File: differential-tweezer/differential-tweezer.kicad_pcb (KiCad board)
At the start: 4 copper layers, 32 x 23 mm, 64 parts, among them J1 5V, J2 IN+, J3 Conn_Coaxial, J4 IN-, J5 Power, U1 R1283B, U2 OPA810, U3 OPA810, U4 OPA810

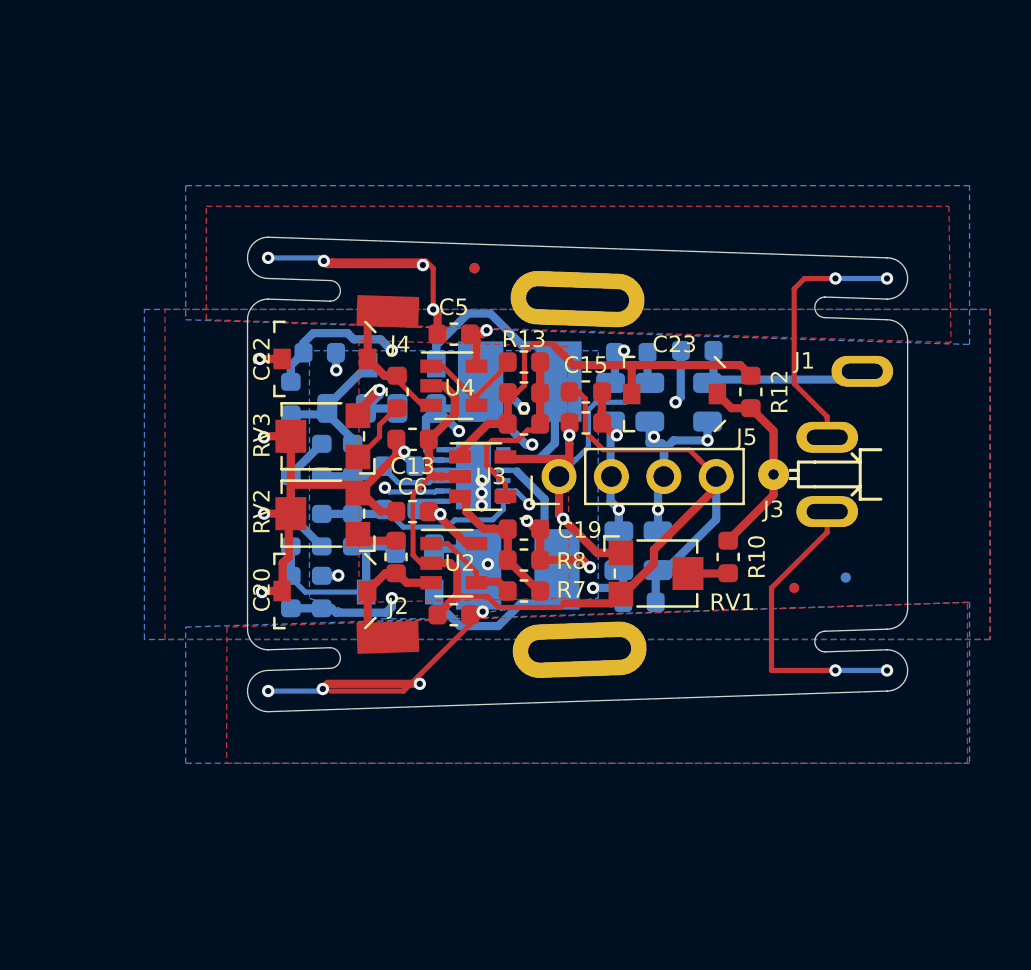
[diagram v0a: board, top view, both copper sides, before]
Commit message: Revision 2
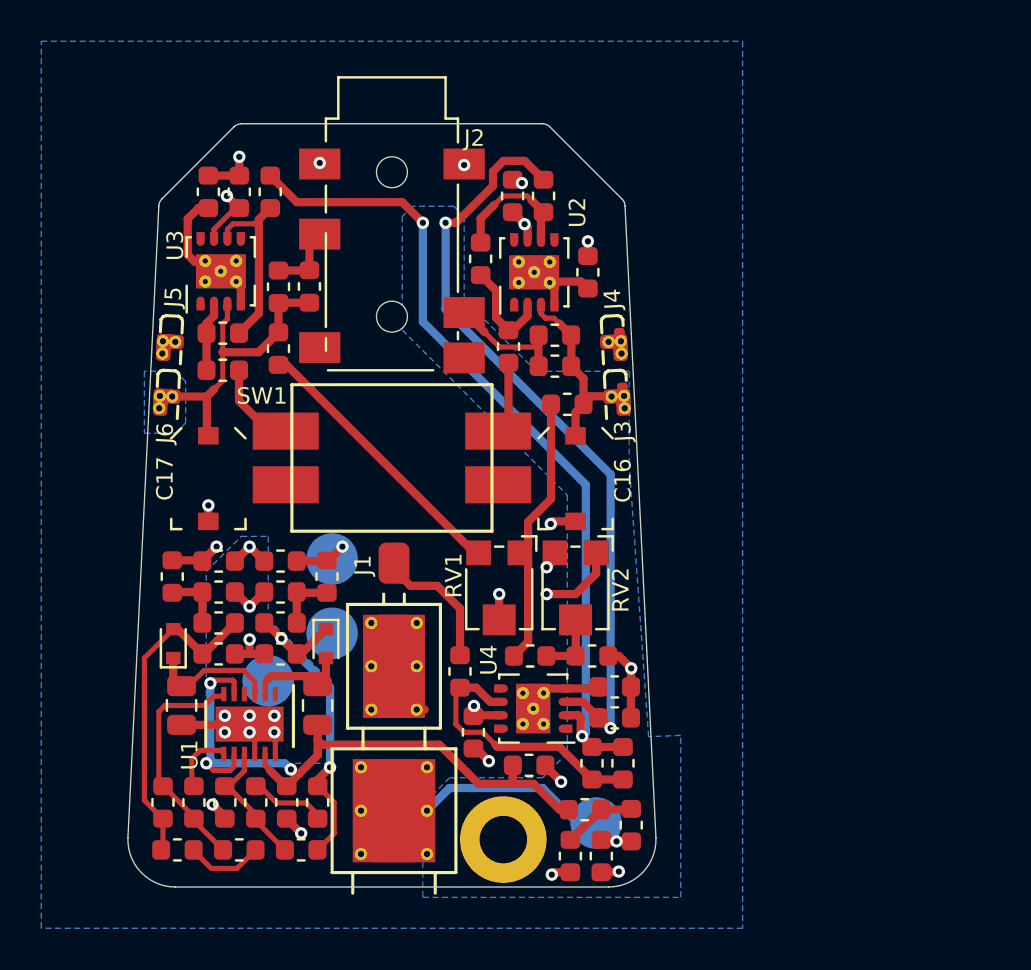
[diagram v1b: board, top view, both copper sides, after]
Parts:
- removed C11: 100nF, Capacitor_SMD:C_0603_1608Metric
- removed C18: 22nF, Capacitor_SMD:C_0603_1608Metric
- removed FID1, FID2, FID3, FID4: Fiducial_0.5mm_Mask1mm, Fiducial:Fiducial_0.5mm_Mask1mm
- removed R8: 470, Resistor_SMD:R_0603_1608Metric
- removed RV3: 47k, Potentiometer_SMD:Potentiometer_Bourns_TC33X_Vertical
- removed SLOT1, SLOT2: SLOT_5x1, oscilloscope-probes:SLOT_5x1
- added C24: 100nF, Capacitor_SMD:C_0603_1608Metric, F.Cu at (88.0, 144.5)
- added C25: 100nF, Capacitor_SMD:C_0603_1608Metric, F.Cu at (94.8, 142.3)
- added C26: 10µF, Capacitor_SMD:C_0603_1608Metric, F.Cu at (78.9, 147.9)
- added H1: 2.2mm, MountingHole:MountingHole_2.2mm_M2_DIN965_Pad, F.Cu at (89.4, 149.7)
- added J6: Probe-, oscilloscope-probes:TE_2306454_LEFT, F.Cu at (72.9, 128.2)
- added L8: 1k, Inductor_SMD:L_0603_1608Metric, F.Cu at (73.3, 136.9)
- added R16: 22, Resistor_SMD:R_0603_1608Metric, F.Cu at (89.7, 125.8)
- added R17: 22, Resistor_SMD:R_0603_1608Metric, F.Cu at (75.8, 127.0)
- added R18: 110, Resistor_SMD:R_0603_1608Metric, F.Cu at (91.3, 118.5)
- added R19: 110, Resistor_SMD:R_0603_1608Metric, F.Cu at (78.1, 118.3)
- added R20: 220, Resistor_SMD:R_0603_1608Metric, F.Cu at (94.8, 143.8)
- added R21: 220, Resistor_SMD:R_0603_1608Metric, F.Cu at (93.7, 146.0)
- added R22: 49.9, Resistor_SMD:R_0603_1608Metric, F.Cu at (87.3, 141.6)
- added SW1: GAIN, oscilloscope-probes:78HF01GWRT, F.Cu at (84.0, 131.2)
- added TP1: +5V, TestPoint:TestPoint_Pad_D2.5mm, B.Cu at (93.9, 148.9)
- added TP2: +6V, TestPoint:TestPoint_Pad_D2.5mm, B.Cu at (81.1, 136.1)
- added TP3: -6V, TestPoint:TestPoint_Pad_D2.5mm, B.Cu at (81.1, 139.7)
- added TP4: GND, TestPoint:TestPoint_Pad_D2.5mm, B.Cu at (78.0, 142.0)
- C1, C12, C2, C9: footprint Capacitor_SMD:C_0805_2012Metric -> Capacitor_SMD:C_0603_1608Metric; moved to F.Cu
- C10: value 10µF -> 100nF; footprint Capacitor_SMD:C_0805_2012Metric -> Capacitor_SMD:C_0603_1608Metric; moved to F.Cu
- C13, C6, C7: value 100nF -> 10µF
- C14, C15: value 100nF -> 20pF
- C16, C17: value 10µF -> 8-30pF; footprint Capacitor_SMD:C_0805_2012Metric -> Capacitor_SMD:C_Trimmer_Murata_TZC3; moved to F.Cu
- C19: value 2pF -> N/A
- C20, C22, C23: value 6pF -> 100nF; footprint Capacitor_SMD:C_Trimmer_Murata_TZC3 -> Capacitor_SMD:C_0603_1608Metric
- C21: value 2pF -> 100nF
- C3: value 100nF -> 10µF; moved to F.Cu
- C4: value 10µF -> 100pF; footprint Capacitor_SMD:C_0805_2012Metric -> Capacitor_SMD:C_0603_1608Metric; moved to F.Cu
- C5: value 100nF -> 100pF
- C8: value 22nF -> 10µF; moved to F.Cu
- D1, D2: value BAT54 -> NSR05T30; footprint Diode_SMD:D_SOD-123 -> Diode_SMD:D_SOD-523; moved to F.Cu
- J1: value 5V -> Triax; footprint oscilloscope-probes:WIREPAD_WIDE -> oscilloscope-probes:TRIAX_TUBE
- J2: value IN+ -> Input; footprint oscilloscope-probes:SOLDERPAD_3x1.5 -> oscilloscope-probes:Tensility_54-00177
- J3: value Conn_Coaxial -> Probe+; footprint oscilloscope-probes:COAX_SOLDER -> oscilloscope-probes:TE_2306454_RIGHT
- J4: value IN- -> Probe+_GND; footprint oscilloscope-probes:SOLDERPAD_3x1.5 -> oscilloscope-probes:TE_2306454_RIGHT
- J5: value Power -> Probe-_GND; footprint Connector_PinHeader_2.54mm:PinHeader_1x04_P2.54mm_Vertical -> oscilloscope-probes:TE_2306454_LEFT
- L1, L5, L6, R1, R4, U1: moved to F.Cu
- L2, L7: value 47µH -> 1k; footprint Inductor_SMD:L_Taiyo-Yuden_NR-40xx_HandSoldering -> Inductor_SMD:L_0603_1608Metric; moved to F.Cu
- L3, L4: value 1k -> 4.7µH; footprint Inductor_SMD:L_0603_1608Metric -> Inductor_SMD:L_0805_2012Metric; moved to F.Cu
- R10, R9: value 1M -> 499k
- R12: value 47 -> 475k
- R13: value 470 -> 475k
- R14: value 470 -> 220
- R15: value 1M -> 220
- R2: value 100k -> 4.99k; moved to F.Cu
- R3: value 10k -> 4.99k; moved to F.Cu
- R5: value 100k -> 1k; moved to F.Cu
- R6: value 10k -> 1k; moved to F.Cu
- R7: value 470 -> 10M
- RV1, RV2: value 47k -> 50k
- U2, U3, U4: value OPA810 -> OPA659; footprint Package_TO_SOT_SMD:SOT-23-5 -> Package_SON:Texas_S-PVSON-N8_ThermalVias
- moved L4 27.7 mm to (73.8, 143.2), turned to 90 degrees
- moved C4 27.2 mm to (77.4, 147.9)
- moved C5 27.1 mm to (76.6, 150.2)
- moved J1 26.1 mm to (84.1, 139.8), turned to 90 degrees
- moved C1 25.0 mm to (94.2, 150.5), turned to 270 degrees
- moved C23 24.6 mm to (75.1, 118.3), turned to 270 degrees
- moved R10 24.2 mm to (80.0, 122.9)
- moved L1 23.2 mm to (95.6, 149.0), turned to 90 degrees
- moved C3 22.4 mm to (90.7, 146.1)
- moved C2 22.1 mm to (92.7, 150.5)
- moved C20 21.2 mm to (89.8, 118.5), turned to 90 degrees
- moved C7 21.0 mm to (75.6, 140.7)
- moved L2 21.0 mm to (93.3, 148.2), turned to 180 degrees
- moved L6 20.4 mm to (75.6, 139.2), turned to 180 degrees
- moved J5 20.1 mm to (73.0, 125.5), turned to 87 degrees
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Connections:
- C1 pad 1: Net-(C1-Pad1) -> +5V
- C10 pad 1: Net-(C10-Pad1) -> /OFFSET_TRIM
- C12 pad 1: -12V -> +6V
- C13 pad 1: GND -> -6V
- C13 pad 2: -12V -> GND
- C14 pad 1: GND -> /IN+
- C14 pad 2: -12V -> /CONN_IN+
- C15 pad 1: GND -> /IN-
- C15 pad 2: -12V -> /CONN_IN-
- C16 pad 1: Net-(C16-Pad1) -> /IN+
- C17 pad 1: Net-(C17-Pad1) -> /IN-
- C19 pad 1: GND -> Net-(C19-Pad1)
- C20 pad 1: Net-(C20-Pad1) -> +6V
- C21 pad 1: Net-(C21-Pad1) -> GND
- C21 pad 2: Net-(C21-Pad2) -> -6V
- C22 pad 1: Net-(C22-Pad1) -> +6V
- C23 pad 1: Net-(C23-Pad1) -> GND
- C23 pad 2: Net-(C21-Pad1) -> -6V
- C3 pad 1: Net-(C2-Pad1) -> Net-(C26-Pad1)
- C4 pad 1: +12V -> Net-(C4-Pad1)
- C4 pad 2: GND -> Net-(C4-Pad2)
- C5 pad 1: +12V -> Net-(C5-Pad1)
- C5 pad 2: GND -> Net-(C5-Pad2)
- C6 pad 1: +12V -> Net-(C6-Pad1)
- C7 pad 1: +12V -> Net-(C7-Pad1)
- C8 pad 2: Net-(C8-Pad2) -> GND
- D1 pad 1: Net-(C1-Pad1) -> Net-(D1-Pad1)
- D1 pad 2: Net-(D1-Pad2) -> Net-(C7-Pad1)
- D2 pad 1: Net-(D2-Pad1) -> Net-(C6-Pad1)
- D2 pad 2: Net-(C9-Pad1) -> Net-(D2-Pad2)
- J1 pad 1: Net-(C16-Pad1) -> /OUT
- J3 pad 1: Net-(C23-Pad1) -> /IN+
- J4 pad 1: Net-(C22-Pad1) -> GND
- J5 pad 1: +12V -> GND
- L1 pad 1: Net-(C16-Pad1) -> +5V
- L1 pad 2: Net-(C17-Pad1) -> Net-(C2-Pad1)
- L2 pad 1: Net-(C17-Pad1) -> Net-(C2-Pad1)
- L2 pad 2: Net-(D1-Pad2) -> Net-(C26-Pad1)
- L3 pad 1: Net-(C1-Pad1) -> Net-(C26-Pad1)
- L3 pad 2: Net-(C2-Pad1) -> Net-(D2-Pad2)
- L4 pad 1: Net-(C2-Pad1) -> GND
- L4 pad 2: +12V -> Net-(D1-Pad1)
- L5 pad 1: Net-(C9-Pad1) -> Net-(C6-Pad1)
- L5 pad 2: Net-(C10-Pad1) -> Net-(C8-Pad1)
- L6 pad 1: Net-(C10-Pad1) -> Net-(C7-Pad1)
- L6 pad 2: -12V -> Net-(C9-Pad1)
- L7 pad 1: GND -> Net-(C8-Pad1)
- L7 pad 2: Net-(D2-Pad1) -> +6V
- R1 pad 1: Net-(C8-Pad1) -> Net-(C5-Pad2)
- R1 pad 2: Net-(C1-Pad1) -> Net-(R1-Pad2)
- R10 pad 1: Net-(R10-Pad1) -> /IN-
- R10 pad 2: Net-(C23-Pad1) -> /CONN_IN-
- R12 pad 1: Net-(C23-Pad1) -> /IN+
- R12 pad 2: Net-(C21-Pad1) -> Net-(R12-Pad2)
- R13 pad 1: Net-(R13-Pad1) -> /IN-
- R13 pad 2: Net-(C21-Pad2) -> Net-(R13-Pad2)
- R14 pad 1: Net-(C21-Pad2) -> Net-(R14-Pad1)
- R14 pad 2: Net-(C21-Pad1) -> Net-(R14-Pad2)
- R15 pad 1: Net-(C22-Pad1) -> Net-(R15-Pad1)
- R2 pad 1: Net-(C1-Pad1) -> Net-(C6-Pad1)
- R2 pad 2: Net-(C8-Pad2) -> Net-(C4-Pad2)
- R3 pad 1: GND -> Net-(C7-Pad1)
- R3 pad 2: Net-(C8-Pad2) -> Net-(C5-Pad2)
- R4 pad 1: Net-(C18-Pad1) -> Net-(C4-Pad1)
- R4 pad 2: Net-(C9-Pad1) -> Net-(C6-Pad1)
- R5 pad 1: Net-(C9-Pad1) -> Net-(C5-Pad1)
- R5 pad 2: Net-(C18-Pad2) -> Net-(C7-Pad1)
- R6 pad 1: Net-(C18-Pad2) -> GND
- R6 pad 2: Net-(R6-Pad2) -> Net-(C4-Pad2)
- R7 pad 1: Net-(R7-Pad1) -> /OFFSET_TRIM
- R7 pad 2: Net-(C19-Pad2) -> Net-(R12-Pad2)
- R9 pad 1: Net-(C20-Pad1) -> /IN+
- R9 pad 2: Net-(R9-Pad2) -> /CONN_IN+
- RV1 pad 1: +12V -> Net-(R12-Pad2)
- RV1 pad 2: Net-(R10-Pad1) -> GND
- RV1 pad 3: -12V -> Net-(R13-Pad2)
- RV2 pad 1: Net-(R9-Pad2) -> +6V
- RV2 pad 2: GND -> /OFFSET_TRIM
- RV2 pad 3: GND -> -6V
- U1 pad 11: Net-(C17-Pad1) -> Net-(C26-Pad1)
- U1 pad 2: Net-(D1-Pad2) -> Net-(D2-Pad2)
- U1 pad 3: Net-(D2-Pad1) -> Net-(D1-Pad1)
- U1 pad 5: Net-(C17-Pad1) -> Net-(C26-Pad1)
- U1 pad 6: Net-(C18-Pad2) -> Net-(C5-Pad2)
- U1 pad 7: Net-(R6-Pad2) -> Net-(R1-Pad2)
- U1 pad 8: Net-(C17-Pad1) -> Net-(C26-Pad1)
- U1 pad 9: Net-(C8-Pad2) -> Net-(C4-Pad2)
- U2 pad 1: Net-(R7-Pad1) -> Net-(U2-Pad1)
- U2 pad 2: -12V -> Net-(R14-Pad2)
- U2 pad 3: Net-(C20-Pad1) -> /IN+
- U2 pad 4: Net-(R7-Pad1) -> -6V
- U2 pad 5: +12V -> Net-(U2-Pad5)
- U3 pad 1: Net-(C21-Pad1) -> Net-(U3-Pad1)
- U3 pad 2: -12V -> Net-(R15-Pad1)
- U3 pad 3: Net-(C19-Pad2) -> /IN-
- U3 pad 4: Net-(C21-Pad2) -> -6V
- U3 pad 5: +12V -> Net-(U3-Pad5)
- U4 pad 1: Net-(R13-Pad1) -> Net-(U4-Pad1)
- U4 pad 2: -12V -> Net-(C19-Pad2)
- U4 pad 3: Net-(C22-Pad1) -> Net-(R18-Pad2)
- U4 pad 4: Net-(R13-Pad1) -> -6V
- U4 pad 5: +12V -> Net-(U4-Pad5)
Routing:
- net GND: track 131.9 -> 34.9 mm, vias 31 -> 24
- net -12V: track 50.4 -> 0.00 mm
- net +12V: track 40.2 -> 0.00 mm, vias 4 -> 0
- net Net-(C17-Pad1): track 38.1 -> 0.00 mm, vias 6 -> 0
- net Net-(R18-Pad2): track 0.00 -> 37.3 mm, vias 0 -> 2
- net Net-(C19-Pad2): track 7.11 -> 41.2 mm, vias 0 -> 2
- net Net-(C26-Pad1): track 0.00 -> 33.1 mm, vias 0 -> 3
- net Net-(C21-Pad1): track 20.4 -> 0.00 mm
- net Net-(C10-Pad1): track 19.3 -> 0.00 mm, vias 2 -> 0
- net Net-(C2-Pad1): track 20.7 -> 3.57 mm, vias 2 -> 0
- net Net-(C6-Pad1): track 0.00 -> 16.2 mm, vias 0 -> 2
- net Net-(C7-Pad1): track 0.00 -> 16.0 mm
- net Net-(D1-Pad2): track 15.4 -> 0.00 mm
- net Net-(D2-Pad1): track 15.3 -> 0.00 mm
- net -6V: track 0.00 -> 14.6 mm, vias 0 -> 2
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- added copper zone on In2.Cu, net +6V
- added copper zone on B.Cu, net -6V
- removed copper zone on F.Cu, net GND
- removed copper zone on In2.Cu, net GND
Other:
- board size 32 x 23 mm -> 25.6 x 37 mm
- rule pad_to_mask_clearance: 0.05 -> 0
- board text added: "Diff. amp devEmbedded Rev 2, 5/2021"
- board text added: "Enclosure front edge"
- board text removed: "+12V"
- board text removed: "+5V"
- board text removed: "-12V"
- board text removed: "Diff. Amp"
- board text removed: "GND"
- board text removed: "JLCJLCJLCJLC"
- board text removed: "Rev 1 01/2021"

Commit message: Revision 3
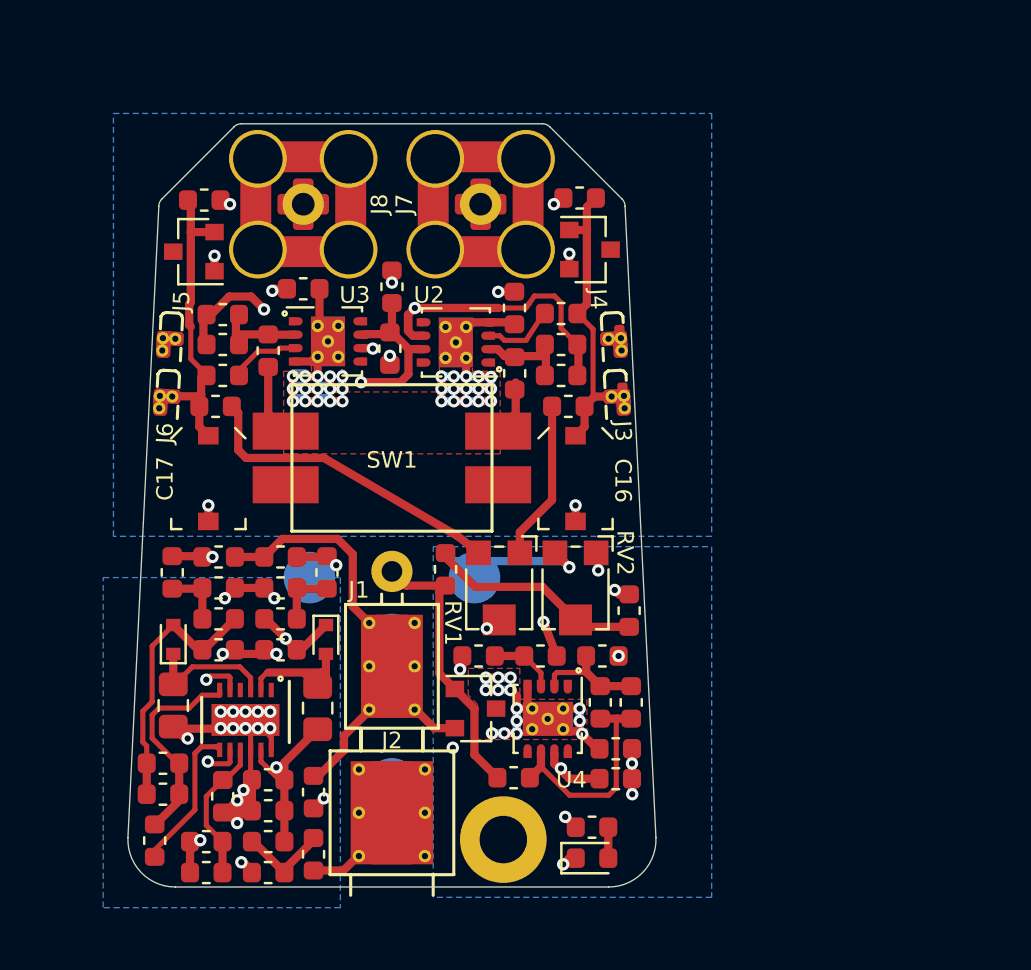
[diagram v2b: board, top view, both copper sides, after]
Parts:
- removed C14, C15: 20pF, Capacitor_SMD:C_0603_1608Metric
- removed R4, R5: 1k, Resistor_SMD:R_0603_1608Metric
- added C11: 3pF, Capacitor_SMD:C_0603_1608Metric, F.Cu at (75.8, 125.7)
- added D3: RED, LED_SMD:LED_0603_1608Metric, F.Cu at (93.7, 150.6)
- added D4: PESD5V0X1B, Package_TO_SOT_SMD:SOT-23, F.Cu at (93.6, 121.1)
- added D5: PESD5V0X1B, Package_TO_SOT_SMD:SOT-23, F.Cu at (74.4, 121.2)
- added D6: PESD5V0X1B, Package_TO_SOT_SMD:SOT-23, F.Cu at (88.0, 143.3)
- added J7: IN+, oscilloscope-probes:RF11-27A-T-00-50-G, F.Cu at (88.3, 118.9)
- added J8: IN-, oscilloscope-probes:RF11-27A-T-00-50-G, F.Cu at (79.7, 118.9)
- added L9: MMZ1608B601, Inductor_SMD:L_0603_1608Metric, F.Cu at (80.2, 147.4)
- added R11: 110, Resistor_SMD:R_0603_1608Metric, F.Cu at (75.8, 127.2)
- added R23: 110, Resistor_SMD:R_0603_1608Metric, F.Cu at (92.2, 124.2)
- added R8: 5.1k, Resistor_SMD:R_0603_1608Metric, F.Cu at (93.7, 149.1)
- C1: value 10µF -> 3pF
- C19: value N/A -> 3pF
- J1: value Triax -> Triax_inner; footprint oscilloscope-probes:TRIAX_TUBE -> oscilloscope-probes:COAX_2MM
- J2: value Input -> Triax_outer; footprint oscilloscope-probes:Tensility_54-00177 -> oscilloscope-probes:TRIAX_OUTER_3MM
- J3: value Probe+ -> Spring+S
- J4: value Probe+_GND -> Spring+G
- J5: value Probe-_GND -> Spring-G
- J6: value Probe- -> Spring-S
- L1, L2, L5, L6, L7, L8: value 1k -> MMZ1608B601
- L3, L4: footprint Inductor_SMD:L_0805_2012Metric -> Inductor_SMD:L_0805_2012Metric_Pad1.15x1.40mm_HandSolder
- R10, R9: value 499k -> 49.9
- R12, R13: value 475k -> 487k
- R16, R17: value 22 -> 24
- R2, R3: value 4.99k -> 5.1k
- R7: value 10M -> 5.1k
- RV1, RV2: value 50k -> 20k
- U1: value R1283B -> R1283K001C
- moved R19 27.7 mm to (94.2, 140.8), turned to 180 degrees
- moved J2 27.4 mm to (84.0, 148.4), turned to 90 degrees
- moved C1 24.9 mm to (92.2, 125.7), turned to 0 degrees
- moved R18 22.3 mm to (91.2, 140.8), turned to 180 degrees
- moved C23 15.9 mm to (89.9, 123.9)
- moved L1 15.5 mm to (80.2, 150.4)
- moved L2 15.4 mm to (78.0, 149.8), turned to 0 degrees
- moved C2 14.7 mm to (78.0, 151.3), turned to 180 degrees
- moved C21 13.8 mm to (79.7, 123.0), turned to 0 degrees
- moved C3 12.7 mm to (78.0, 146.8), turned to 180 degrees
- moved C22 10.5 mm to (83.9, 125.9), turned to 270 degrees
- moved TP1 10.1 mm to (84.0, 147.0)
- moved TP3 7.41 mm to (88.0, 137.0)
- moved C20 7.32 mm to (84.0, 122.9)
- moved C24 7.26 mm to (94.8, 146.8), turned to 0 degrees
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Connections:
- C1 pad 1: +5V -> Net-(C1-Pad1)
- C1 pad 2: GND -> Net-(C1-Pad2)
- C10 pad 2: GND -> GNDA
- C12 pad 2: GND -> GNDA
- C13 pad 2: GND -> GNDA
- C16 pad 2: GND -> GNDA
- C17 pad 2: GND -> GNDA
- C20 pad 2: GND -> GNDA
- C21 pad 1: GND -> GNDA
- C22 pad 2: GND -> GNDA
- C23 pad 1: GND -> GNDA
- C24 pad 2: GND -> GNDA
- C25 pad 1: GND -> GNDA
- C6 pad 1: Net-(C6-Pad1) -> Net-(C4-Pad1)
- C7 pad 1: Net-(C7-Pad1) -> Net-(C5-Pad1)
- D1 pad 2: Net-(C7-Pad1) -> Net-(C5-Pad1)
- D2 pad 1: Net-(C6-Pad1) -> Net-(C4-Pad1)
- H1 pad 1: GND -> GNDA
- J1 pad 2: GND -> GNDA
- J4 pad 1: GND -> GNDA
- J5 pad 1: GND -> GNDA
- L5 pad 1: Net-(C6-Pad1) -> Net-(C4-Pad1)
- L6 pad 1: Net-(C7-Pad1) -> Net-(C5-Pad1)
- R14 pad 1: Net-(R14-Pad1) -> Net-(C1-Pad2)
- R14 pad 2: Net-(R14-Pad2) -> Net-(C1-Pad1)
- R15 pad 1: Net-(R15-Pad1) -> Net-(C11-Pad2)
- R16 pad 1: Net-(R16-Pad1) -> Net-(C1-Pad1)
- R16 pad 2: Net-(R14-Pad2) -> Net-(R16-Pad2)
- R17 pad 1: Net-(R17-Pad1) -> Net-(C11-Pad2)
- R17 pad 2: Net-(R15-Pad1) -> Net-(R17-Pad2)
- R18 pad 1: Net-(R14-Pad1) -> Net-(C1-Pad2)
- R2 pad 1: Net-(C6-Pad1) -> Net-(C4-Pad1)
- R20 pad 2: GND -> GNDA
- R3 pad 1: Net-(C7-Pad1) -> Net-(C5-Pad1)
- R7 pad 2: Net-(R12-Pad2) -> /OUT
- RV1 pad 2: GND -> GNDA
- SW1 pad 1: Net-(R17-Pad1) -> Net-(R17-Pad2)
- SW1 pad 2: Net-(R16-Pad1) -> Net-(R16-Pad2)
- TP4 pad 1: GND -> GNDA
- U2 pad 2: Net-(R14-Pad2) -> Net-(C1-Pad1)
- U2 pad 3: /IN+ -> Net-(R23-Pad1)
- U2 pad 6: Net-(R14-Pad1) -> Net-(C1-Pad2)
- U3 pad 2: Net-(R15-Pad1) -> Net-(C11-Pad2)
- U3 pad 3: /IN- -> Net-(R11-Pad1)
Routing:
- net -6V: track 14.6 -> 75.5 mm, vias 2 -> 47
- net GNDA: track 0.00 -> 51.1 mm, vias 0 -> 14
- net +6V: track 13.9 -> 64.5 mm
- net Net-(C19-Pad2): track 41.2 -> 5.42 mm, vias 2 -> 0
- net Net-(R18-Pad2): track 37.3 -> 3.06 mm, vias 2 -> 0
- net Net-(C1-Pad2): track 0.00 -> 33.9 mm, vias 0 -> 2
- net Net-(C11-Pad1): track 9.67 -> 32.9 mm, vias 0 -> 3
- net Net-(C6-Pad1): track 16.2 -> 0.00 mm, vias 2 -> 0
- net Net-(C7-Pad1): track 16.0 -> 0.00 mm
- net Net-(C4-Pad1): track 3.65 -> 19.5 mm, vias 0 -> 2
- net Net-(C26-Pad1): track 33.1 -> 20.7 mm
- net Net-(C5-Pad1): track 3.77 -> 13.0 mm
- net /OFFSET_TRIM: track 3.18 -> 10.5 mm
- net /OUT: track 6.55 -> 13.5 mm
- net Net-(R14-Pad1): track 6.41 -> 0.00 mm
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- added copper zone on F.Cu, net -6V
- added copper zone on In1.Cu, net -6V
- added copper zone on In2.Cu, net GND
- added copper zone on In2.Cu, net GNDA
- removed copper zone on In2.Cu, net +6V
- removed copper zone on In1.Cu, net GND
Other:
- board text added: "DEDP-100 Rev 3, 6/2021"
- board text added: "Main pcb front edge"
- board text removed: "Diff. amp devEmbedded Rev 2, 5/2021"
- board text removed: "Enclosure front edge"
